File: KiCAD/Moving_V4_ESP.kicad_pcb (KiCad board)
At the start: 2 copper layers, 39 x 63 mm, 89 parts, among them J1 Vin_1, J10 IO27_GPIO1, J11 IO32_GPIO2, J12 IO5_GPIO3(PU), J2 Power_SW, J3 Vin_XT, J4 USB_B_Micro, J5 Encorder_L, J6 Encorder_R, J7 MOTOR_L, J8 MOTOR_R, J9 IO4_GPIO0, Q1 U4_ALT2, Q2 U4_ALT2, Q3 U4_ALT2, U1 CN39033A, U10 ITR8307-S17-TR8, U2 CH340X, U3 UZ1085L-33-TN3-R, U4 TXB0104RUT, U5 CP3119MDTR, U6 CP3119MDTR, U7 ESP32-WROOM-32, U8 ITR8307-S17-TR8, U9 ITR8307-S17-TR8

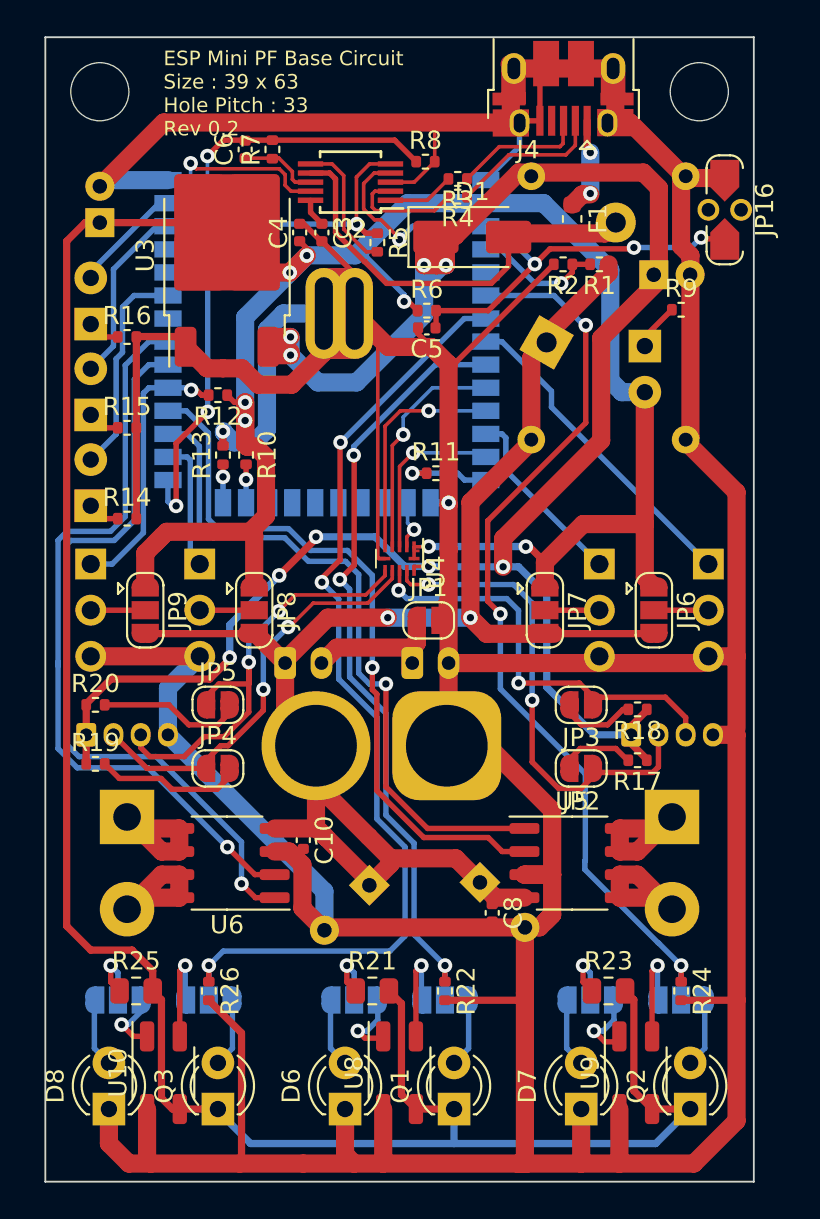
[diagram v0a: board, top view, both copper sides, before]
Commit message: 基本的なシルクを配置
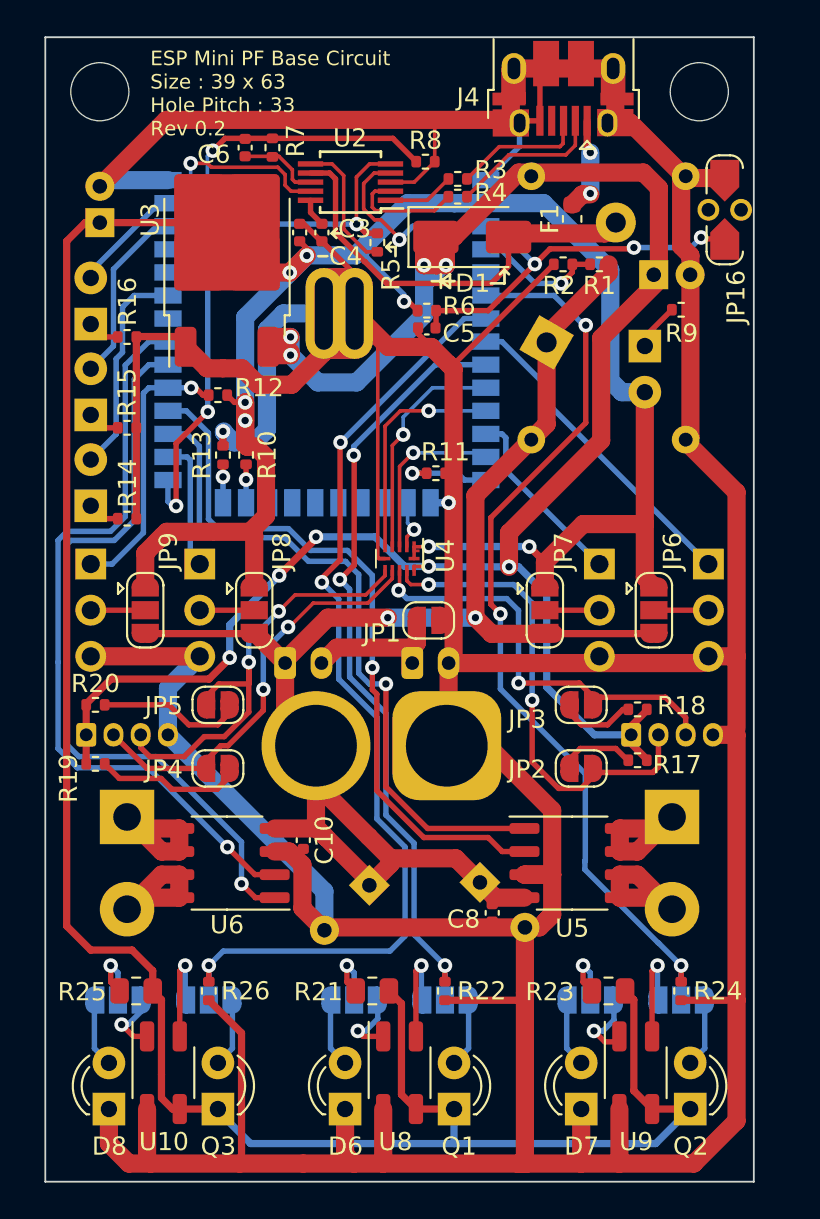
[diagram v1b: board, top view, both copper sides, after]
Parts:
- moved C6 0.10 mm to (111.0, 106.1)
- moved R7 0.10 mm to (112.5, 106.1)
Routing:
- net GND: track 380.8 -> 375.3 mm
- net +5V: track 114.6 -> 112.3 mm
- net /EN: track 33.6 -> 33.0 mm
- net Net-(J6-Pin_3): track 26.0 -> 25.3 mm
- net /Vin: track 88.6 -> 88.0 mm
